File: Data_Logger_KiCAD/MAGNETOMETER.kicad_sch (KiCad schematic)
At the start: 3 parts, among them U11 MMC5983MA

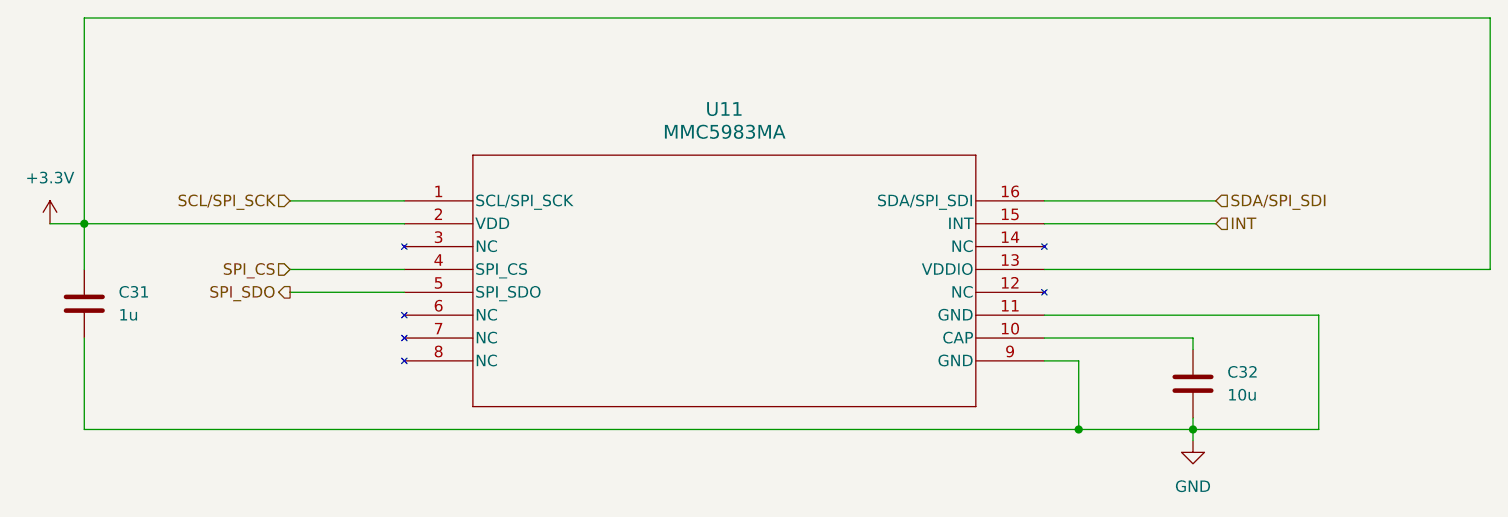
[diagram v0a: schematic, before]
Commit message: Magnetometer Footprint Added
Magnetometer Footprint Added
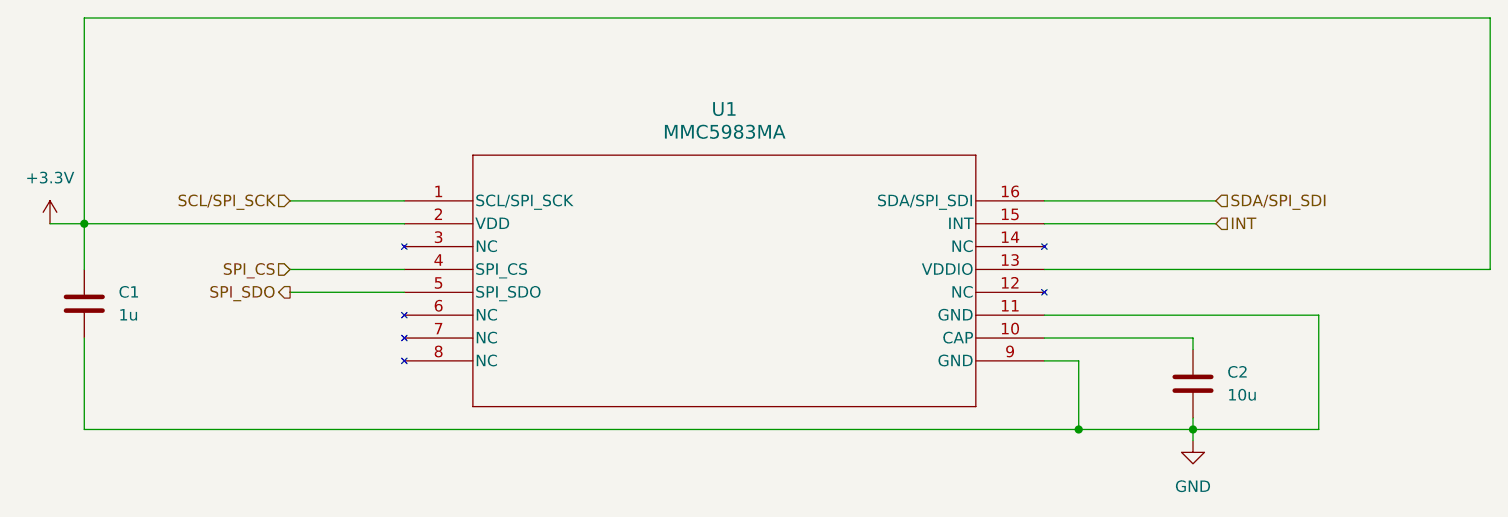
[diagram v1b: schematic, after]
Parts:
- U1: renamed from U11; footprint footprints:MMC5983MA_MEM -> MMC5983MA:MMC5983MA_MEM
- renumbered C31 to C1, C32 to C2
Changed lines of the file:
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@@
 		(dnp no)
 		(fields_autoplaced yes)
-		(property "Reference" "C32"
+		(property "Reference" "C2"
 			(at 191.77 81.2799 0)
 			(effects
@@
 		)
 		(instances
+			(project "MAGNETOMETER"
+				(path "/b7fc4674-3df6-4f05-a8d1-6eebc1d35db8"
+					(reference "C2")
+					(unit 1)
+				)
+			)
 			(project "Data_Logger_Board"
 				(path "/db968e42-3ace-4cc9-9096-9d8f48135c40/795ab2be-9db7-4254-b05c-ac2b60177344/884971b6-34e3-480e-b770-6637cf2c2272"
@@
 		(dnp no)
 		(fields_autoplaced yes)
-		(property "Reference" "#PWR055"
+		(property "Reference" "#PWR0101"
 			(at 60.96 68.58 0)
 			(effects
@@
 		)
 		(instances
+			(project "MAGNETOMETER"
+				(path "/b7fc4674-3df6-4f05-a8d1-6eebc1d35db8"
+					(reference "#PWR0101")
+					(unit 1)
+				)
+			)
 			(project "Data_Logger_Board"
 				(path "/db968e42-3ace-4cc9-9096-9d8f48135c40/795ab2be-9db7-4254-b05c-ac2b60177344/884971b6-34e3-480e-b770-6637cf2c2272"
@@
 		(dnp no)
 		(fields_autoplaced yes)
-		(property "Reference" "#PWR056"
+		(property "Reference" "#PWR0102"
 			(at 187.96 95.25 0)
 			(effects
@@
 		)
 		(instances
+			(project "MAGNETOMETER"
+				(path "/b7fc4674-3df6-4f05-a8d1-6eebc1d35db8"
+					(reference "#PWR0102")
+					(unit 1)
+				)
+			)
 			(project "Data_Logger_Board"
 				(path "/db968e42-3ace-4cc9-9096-9d8f48135c40/795ab2be-9db7-4254-b05c-ac2b60177344/884971b6-34e3-480e-b770-6637cf2c2272"
@@
 		(dnp no)
 		(fields_autoplaced yes)
-		(property "Reference" "U11"
+		(property "Reference" "U1"
 			(at 135.89 52.07 0)
 			(effects
@@
 			)
 		)
-		(property "Footprint" "footprints:MMC5983MA_MEM"
+		(property "Footprint" "MMC5983MA:MMC5983MA_MEM"
 			(at 100.33 62.23 0)
 			(effects
@@
 		)
 		(instances
+			(project "MAGNETOMETER"
+				(path "/b7fc4674-3df6-4f05-a8d1-6eebc1d35db8"
+					(reference "U1")
+					(unit 1)
+				)
+			)
 			(project "Data_Logger_Board"
 				(path "/db968e42-3ace-4cc9-9096-9d8f48135c40/795ab2be-9db7-4254-b05c-ac2b60177344/884971b6-34e3-480e-b770-6637cf2c2272"
@@
 		(dnp no)
 		(fields_autoplaced yes)
-		(property "Reference" "C31"
+		(property "Reference" "C1"
 			(at 68.58 72.3899 0)
 			(effects
@@
 		)
 		(instances
+			(project "MAGNETOMETER"
+				(path "/b7fc4674-3df6-4f05-a8d1-6eebc1d35db8"
+					(reference "C1")
+					(unit 1)
+				)
+			)
 			(project "Data_Logger_Board"
 				(path "/db968e42-3ace-4cc9-9096-9d8f48135c40/795ab2be-9db7-4254-b05c-ac2b60177344/884971b6-34e3-480e-b770-6637cf2c2272"
@@
 		)
 	)
+	(sheet_instances
+		(path "/"
+			(page "1")
+		)
+	)
+	(embedded_fonts no)
 )

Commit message: synced sheet pins in Data_Logger_Board_pro
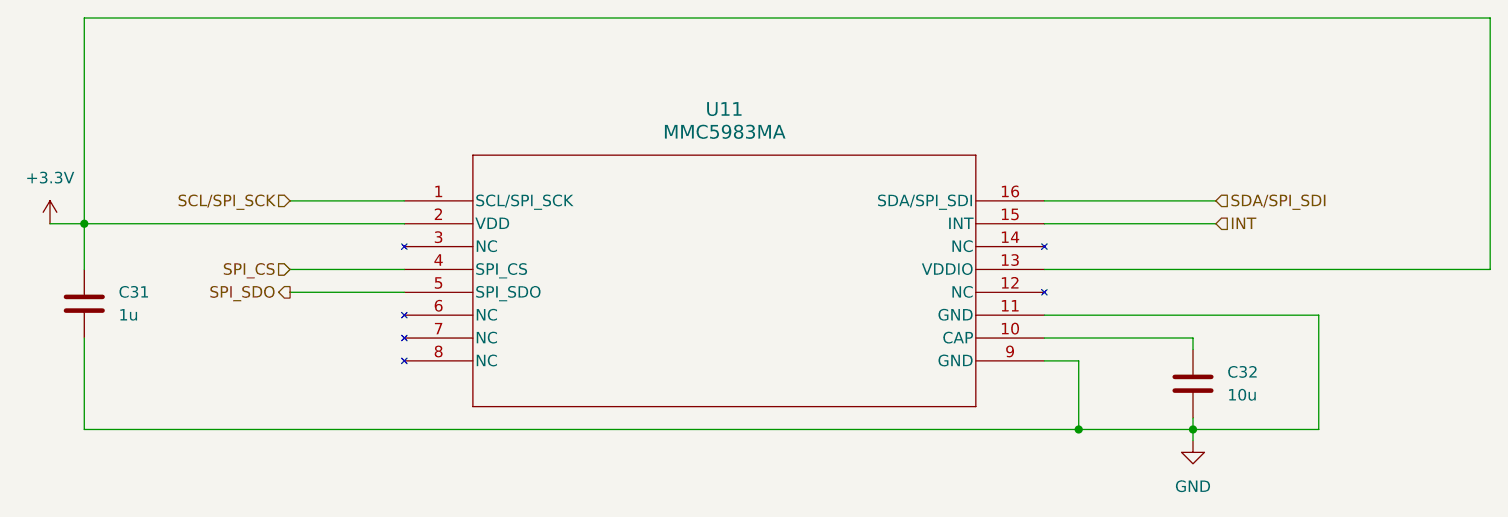
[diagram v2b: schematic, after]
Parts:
- U11: renamed from U1; footprint MMC5983MA:MMC5983MA_MEM -> footprints:MMC5983MA_MEM
- renumbered C1 to C31, C2 to C32
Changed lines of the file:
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@@
 		(dnp no)
 		(fields_autoplaced yes)
-		(property "Reference" "C2"
+		(property "Reference" "C32"
 			(at 191.77 81.2799 0)
 			(effects
@@
 		)
 		(instances
-			(project "MAGNETOMETER"
-				(path "/b7fc4674-3df6-4f05-a8d1-6eebc1d35db8"
-					(reference "C2")
-					(unit 1)
-				)
-			)
 			(project "Data_Logger_Board"
 				(path "/db968e42-3ace-4cc9-9096-9d8f48135c40/795ab2be-9db7-4254-b05c-ac2b60177344/884971b6-34e3-480e-b770-6637cf2c2272"
@@
 		(dnp no)
 		(fields_autoplaced yes)
-		(property "Reference" "#PWR0101"
+		(property "Reference" "#PWR055"
 			(at 60.96 68.58 0)
 			(effects
@@
 		)
 		(instances
-			(project "MAGNETOMETER"
-				(path "/b7fc4674-3df6-4f05-a8d1-6eebc1d35db8"
-					(reference "#PWR0101")
-					(unit 1)
-				)
-			)
 			(project "Data_Logger_Board"
 				(path "/db968e42-3ace-4cc9-9096-9d8f48135c40/795ab2be-9db7-4254-b05c-ac2b60177344/884971b6-34e3-480e-b770-6637cf2c2272"
@@
 		(dnp no)
 		(fields_autoplaced yes)
-		(property "Reference" "#PWR0102"
+		(property "Reference" "#PWR056"
 			(at 187.96 95.25 0)
 			(effects
@@
 		)
 		(instances
-			(project "MAGNETOMETER"
-				(path "/b7fc4674-3df6-4f05-a8d1-6eebc1d35db8"
-					(reference "#PWR0102")
-					(unit 1)
-				)
-			)
 			(project "Data_Logger_Board"
 				(path "/db968e42-3ace-4cc9-9096-9d8f48135c40/795ab2be-9db7-4254-b05c-ac2b60177344/884971b6-34e3-480e-b770-6637cf2c2272"
@@
 		(dnp no)
 		(fields_autoplaced yes)
-		(property "Reference" "U1"
+		(property "Reference" "U11"
 			(at 135.89 52.07 0)
 			(effects
@@
 			)
 		)
-		(property "Footprint" "MMC5983MA:MMC5983MA_MEM"
+		(property "Footprint" "footprints:MMC5983MA_MEM"
 			(at 100.33 62.23 0)
 			(effects
@@
 		)
 		(instances
-			(project "MAGNETOMETER"
-				(path "/b7fc4674-3df6-4f05-a8d1-6eebc1d35db8"
-					(reference "U1")
-					(unit 1)
-				)
-			)
 			(project "Data_Logger_Board"
 				(path "/db968e42-3ace-4cc9-9096-9d8f48135c40/795ab2be-9db7-4254-b05c-ac2b60177344/884971b6-34e3-480e-b770-6637cf2c2272"
@@
 		(dnp no)
 		(fields_autoplaced yes)
-		(property "Reference" "C1"
+		(property "Reference" "C31"
 			(at 68.58 72.3899 0)
 			(effects
@@
 		)
 		(instances
-			(project "MAGNETOMETER"
-				(path "/b7fc4674-3df6-4f05-a8d1-6eebc1d35db8"
-					(reference "C1")
-					(unit 1)
-				)
-			)
 			(project "Data_Logger_Board"
 				(path "/db968e42-3ace-4cc9-9096-9d8f48135c40/795ab2be-9db7-4254-b05c-ac2b60177344/884971b6-34e3-480e-b770-6637cf2c2272"
@@
 		)
 	)
-	(sheet_instances
-		(path "/"
-			(page "1")
-		)
-	)
-	(embedded_fonts no)
 )
